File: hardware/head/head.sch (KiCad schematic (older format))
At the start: 12 parts, among them J1 DB9_Male, J2 Stats_Button, J3 Flush_Button, J4 Brew_Button, J5 Temp_Ok, J6 Display, J7 HX711, J8 Rotary_Encoder, U1 Teensy4.0

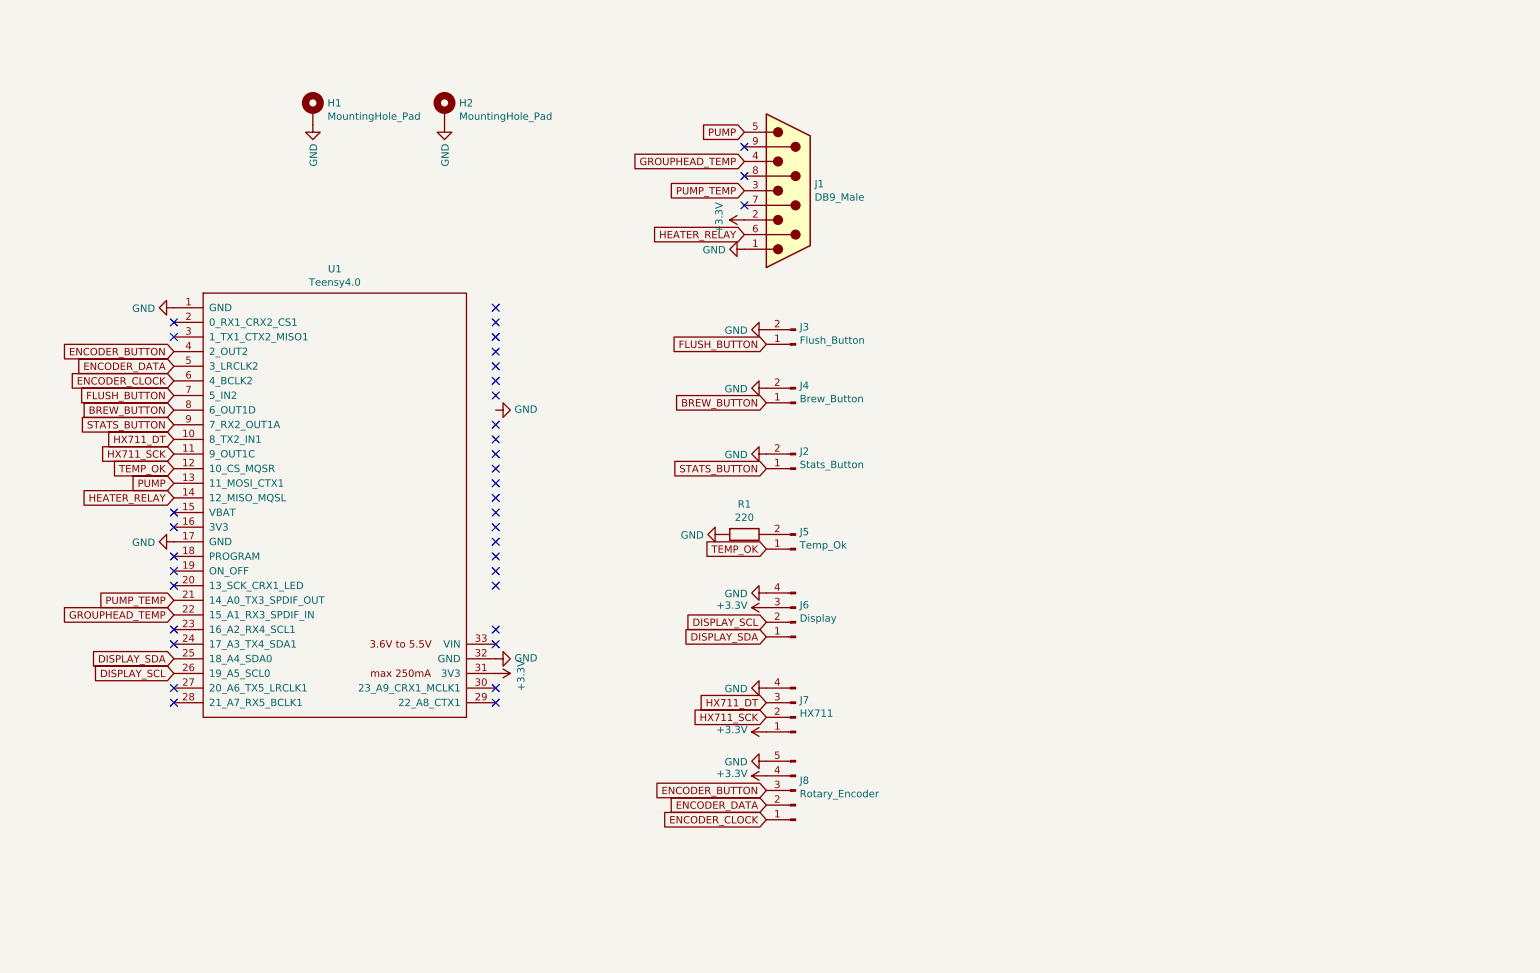
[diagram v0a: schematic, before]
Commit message: Update head unit
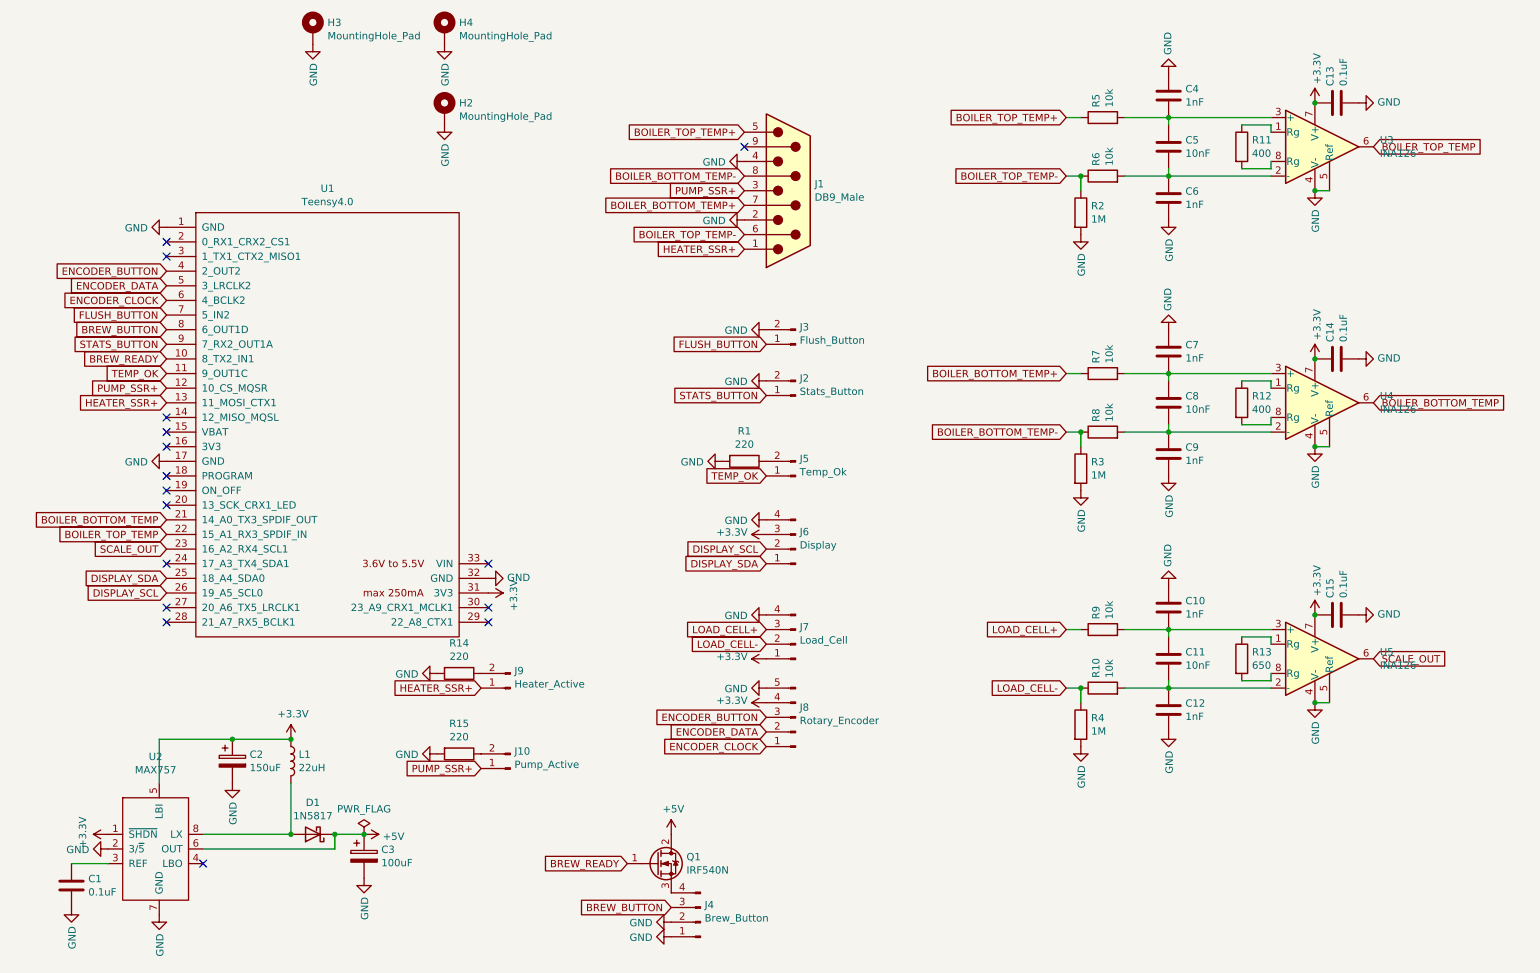
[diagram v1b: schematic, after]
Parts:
- removed H1: MountingHole_Pad, MountingHole:MountingHole_2.5mm_Pad, symbol Mechanical:MountingHole_Pad
- removed J4: Brew_Button, Connector_PinHeader_2.54mm:PinHeader_1x02_P2.54mm_Vertical, symbol Connector:Conn_01x02_Male
- added C1, C13, C14, C15: 0.1uF, Capacitor_THT:C_Disc_D5.1mm_W3.2mm_P5.00mm, symbol Device:C
- added C10, C12, C4, C6, C7, C9: 1nF, Capacitor_THT:C_Disc_D5.1mm_W3.2mm_P5.00mm, symbol Device:C
- added C11, C5, C8: 10nF, Capacitor_THT:C_Disc_D5.1mm_W3.2mm_P5.00mm, symbol Device:C
- added C2: 150uF, Capacitor_THT:CP_Radial_D5.0mm_P2.00mm, symbol Device:CP
- added C3: 100uF, Capacitor_THT:CP_Radial_D5.0mm_P2.00mm, symbol Device:CP
- added D1: 1N5817, Diode_THT:D_DO-41_SOD81_P10.16mm_Horizontal, symbol Diode:1N5817
- added H3, H4: MountingHole_Pad, MountingHole:MountingHole_2.5mm_Pad, symbol Mechanical:MountingHole_Pad
- added J10: Pump_Active, Connector_PinHeader_2.54mm:PinHeader_1x02_P2.54mm_Vertical, symbol Connector:Conn_01x02_Male
- added J4: Brew_Button, Connector_PinHeader_2.54mm:PinHeader_1x04_P2.54mm_Vertical, symbol Connector:Conn_01x04_Male
- added J9: Heater_Active, Connector_PinHeader_2.54mm:PinHeader_1x02_P2.54mm_Vertical, symbol Connector:Conn_01x02_Male
- added L1: 22uH, Inductor_THT:L_Axial_L11.0mm_D4.5mm_P15.24mm_Horizontal_Fastron_MECC, symbol Device:L
- added Q1: IRF540N, Package_TO_SOT_THT:TO-220-3_Vertical, symbol Transistor_FET:IRF540N
- added R10, R5, R6, R7, R8, R9: 10k, Resistor_THT:R_Axial_DIN0204_L3.6mm_D1.6mm_P5.08mm_Horizontal, symbol Device:R
- added R11, R12: 400, Resistor_THT:R_Axial_DIN0204_L3.6mm_D1.6mm_P5.08mm_Horizontal, symbol Device:R
- added R13: 650, Resistor_THT:R_Axial_DIN0204_L3.6mm_D1.6mm_P5.08mm_Horizontal, symbol Device:R
- added R14, R15: 220, Resistor_THT:R_Axial_DIN0204_L3.6mm_D1.6mm_P5.08mm_Horizontal, symbol Device:R
- added R2, R3, R4: 1M, Resistor_THT:R_Axial_DIN0204_L3.6mm_D1.6mm_P5.08mm_Horizontal, symbol Device:R
- added U2: MAX757, Package_DIP:DIP-8_W7.62mm, symbol boost_converter:MAX757
- added U3, U4, U5: INA126, Package_DIP:DIP-8_W7.62mm, symbol Amplifier_Instrumentation:INA128
- J7: value HX711 -> Load_Cell; footprint Connector_RJ:RJ14_Connfly_DS1133-S4_Horizontal -> Connector_PinHeader_2.54mm:PinHeader_1x04_P2.54mm_Vertical
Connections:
- net +3V3: now also C13.1, C14.1, C15.1, C2.1, L1.1, U2.1 (~SHDN), U2.5 (LBI), U3.7 (V+), U4.7 (V+), U5.7 (V+); no longer J1.2
- net BREW_BUTTON: now also J4.3 (Pin_3)
- net GND: now also J1.2, J1.4, C1.2, C10.1, C12.2, C13.2, C14.2, C15.2, C2.2, C3.2, C4.1, C6.2, C7.1, C9.2, H3.1, H4.1, J4.1 (Pin_1), J4.2 (Pin_2), R14.2, R15.2, R2.2, R3.2, R4.2, U2.2 (3/~5), U2.7 (GND), U3.4 (V-), U3.5 (Ref), U4.4 (V-), U4.5 (Ref), U5.4 (V-), U5.5 (Ref); no longer J1.1
- net TEMP_OK: now also U1.11 (9_OUT1C); no longer U1.12 (10_CS_MQSR)
- net BOILER_BOTTOM_TEMP+: now reaches J1.7
- net BOILER_BOTTOM_TEMP+: now also R7.1
- net BOILER_BOTTOM_TEMP-: now reaches J1.8
- net BOILER_BOTTOM_TEMP-: now also R3.1, R8.1
- net SCALE_OUT: now reaches U1.23 (16_A2_RX4_SCL1)
- net SCALE_OUT: now also U5.6
- net GROUPHEAD_TEMP renamed BOILER_TOP_TEMP
- net BOILER_TOP_TEMP: now also U3.6; no longer J1.4
- net HEATER_RELAY: no longer names the net of U1.14 (12_MISO_MQSL)
- net HEATER_RELAY: no longer J1.6
- net HX711_DT renamed BREW_READY
- net BREW_READY: now also Q1.1 (G); no longer J7.3 (Pin_3)
- net HX711_SCK renamed LOAD_CELL-
- net LOAD_CELL-: now also R10.1, R4.1; no longer U1.11 (9_OUT1C)
- net PUMP renamed BOILER_TOP_TEMP+
- net BOILER_TOP_TEMP+: now also R5.1; no longer U1.13 (11_MOSI_CTX1)
- net PUMP_TEMP renamed BOILER_BOTTOM_TEMP
- net BOILER_BOTTOM_TEMP: now also U4.6; no longer J1.3
- new net: R12.1, U4.1 (Rg)
- new net: C8.2, C9.1, R8.2, U4.2 (-)
- new net: C7.2, C8.1, R7.2, U4.3 (+)
- new net: R12.2, U4.8 (Rg)
- new net: R11.1, U3.1 (Rg)
- new net: C5.2, C6.1, R6.2, U3.2 (-)
- new net: C4.2, C5.1, R5.2, U3.3 (+)
- new net: R11.2, U3.8 (Rg)
- new net: R13.1, U5.1 (Rg)
- new net: C11.2, C12.1, R10.2, U5.2 (-)
- new net: C10.2, C11.1, R9.2, U5.3 (+)
- new net: R13.2, U5.8 (Rg)
- new net: C1.1, U2.3 (REF)
- new net: D1.2 (A), L1.2, U2.8 (LX)
- new net: J4.4 (Pin_4), Q1.3 (S)
- new net: J9.2 (Pin_2), R14.1
- new net: J10.2 (Pin_2), R15.1
- new net +5V: C3.1, D1.1 (K), Q1.2 (D), U2.6 (OUT)
- new net BOILER_TOP_TEMP-: J1.6, R2.1, R6.1
- new net HEATER_SSR+: J1.1, J9.1 (Pin_1), U1.13 (11_MOSI_CTX1)
- new net LOAD_CELL+: J7.3 (Pin_3), R9.1
- new net PUMP_SSR+: J1.3, J10.1 (Pin_1), U1.12 (10_CS_MQSR)
- no-connect marks 37 -> 16
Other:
- moved on the sheet: J2, J5, J6, J7, J8, R1, U1
